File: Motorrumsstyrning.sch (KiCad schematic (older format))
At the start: 60 parts, among them J1 SD_Card_Connector, J10 Jumper, J11 Jumper, J12 Jumper, J13 Jumper, J14 Jumper, J15 Jumper, J16 Jumper, J17 Jumper, J18 Jumper, J19 Jumper, J2 Jumper, J20 Jumper, J21 Jumper, J22 Jumper, J23 Screw_Terminal_01x10, J24 Screw_Terminal_01x10, J3 Jumper, J4 Jumper, J5 Jumper, J6 Jumper, J7 Jumper, J8 Jumper, J9 Jumper, Q1 BC337, Q2 BC337, U1 NUCLEO-F303K8, U2 LM1084-5.0, U3 MCP2551-I-P

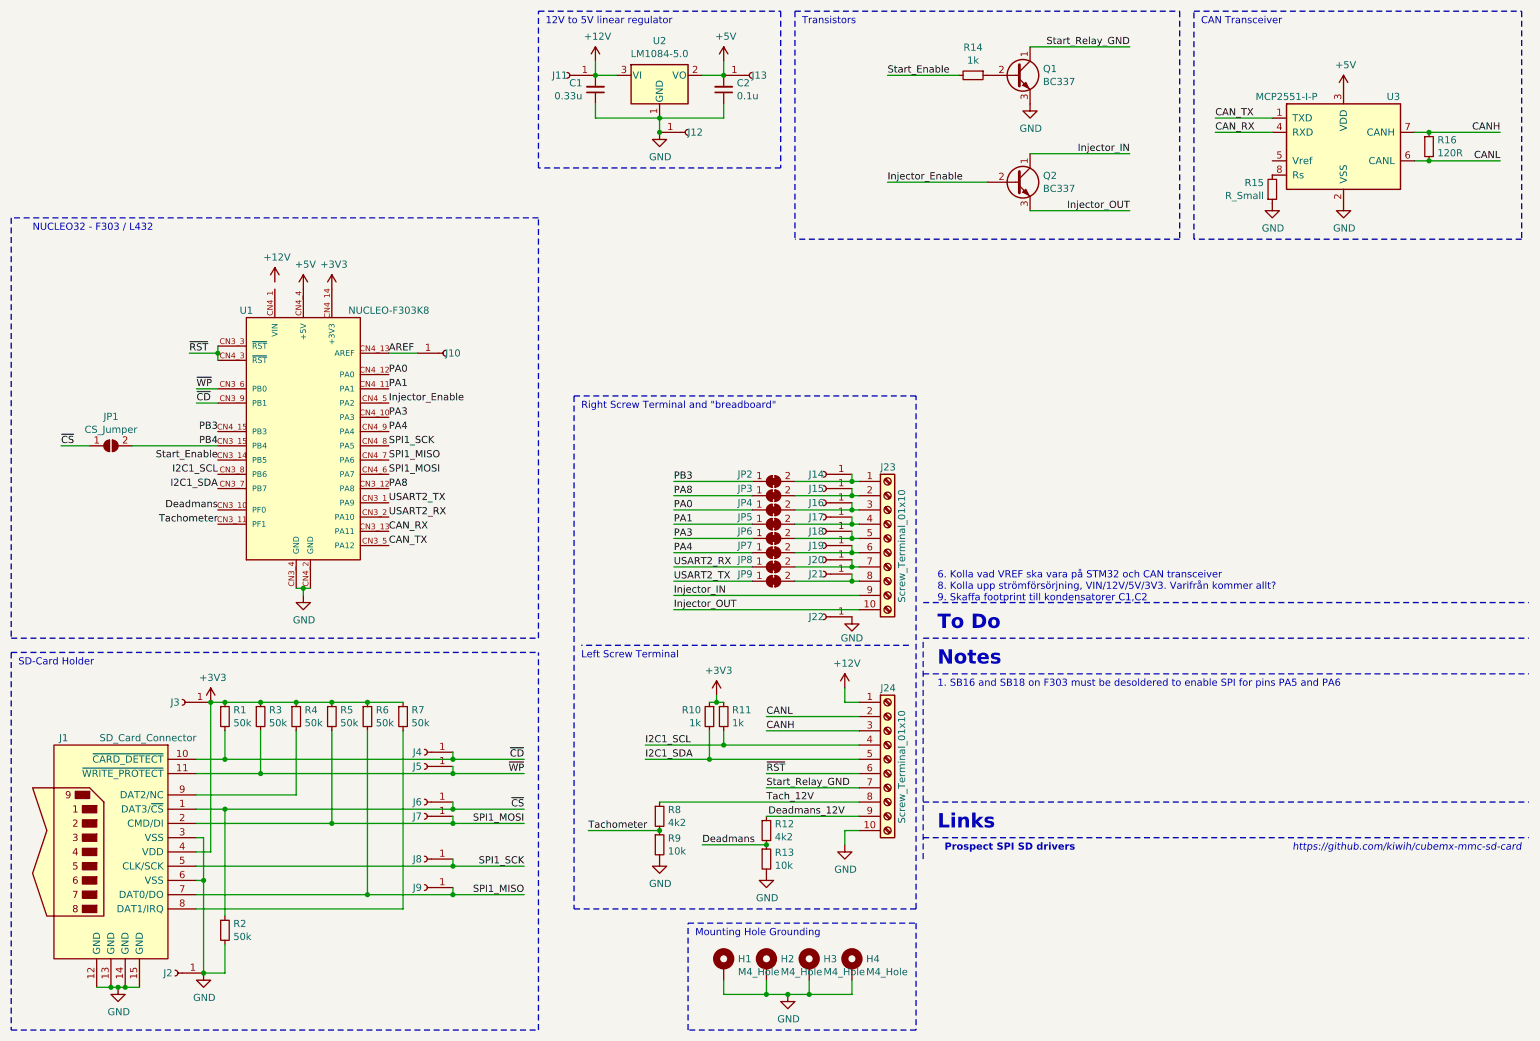
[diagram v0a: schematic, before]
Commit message: Vidareutveckling
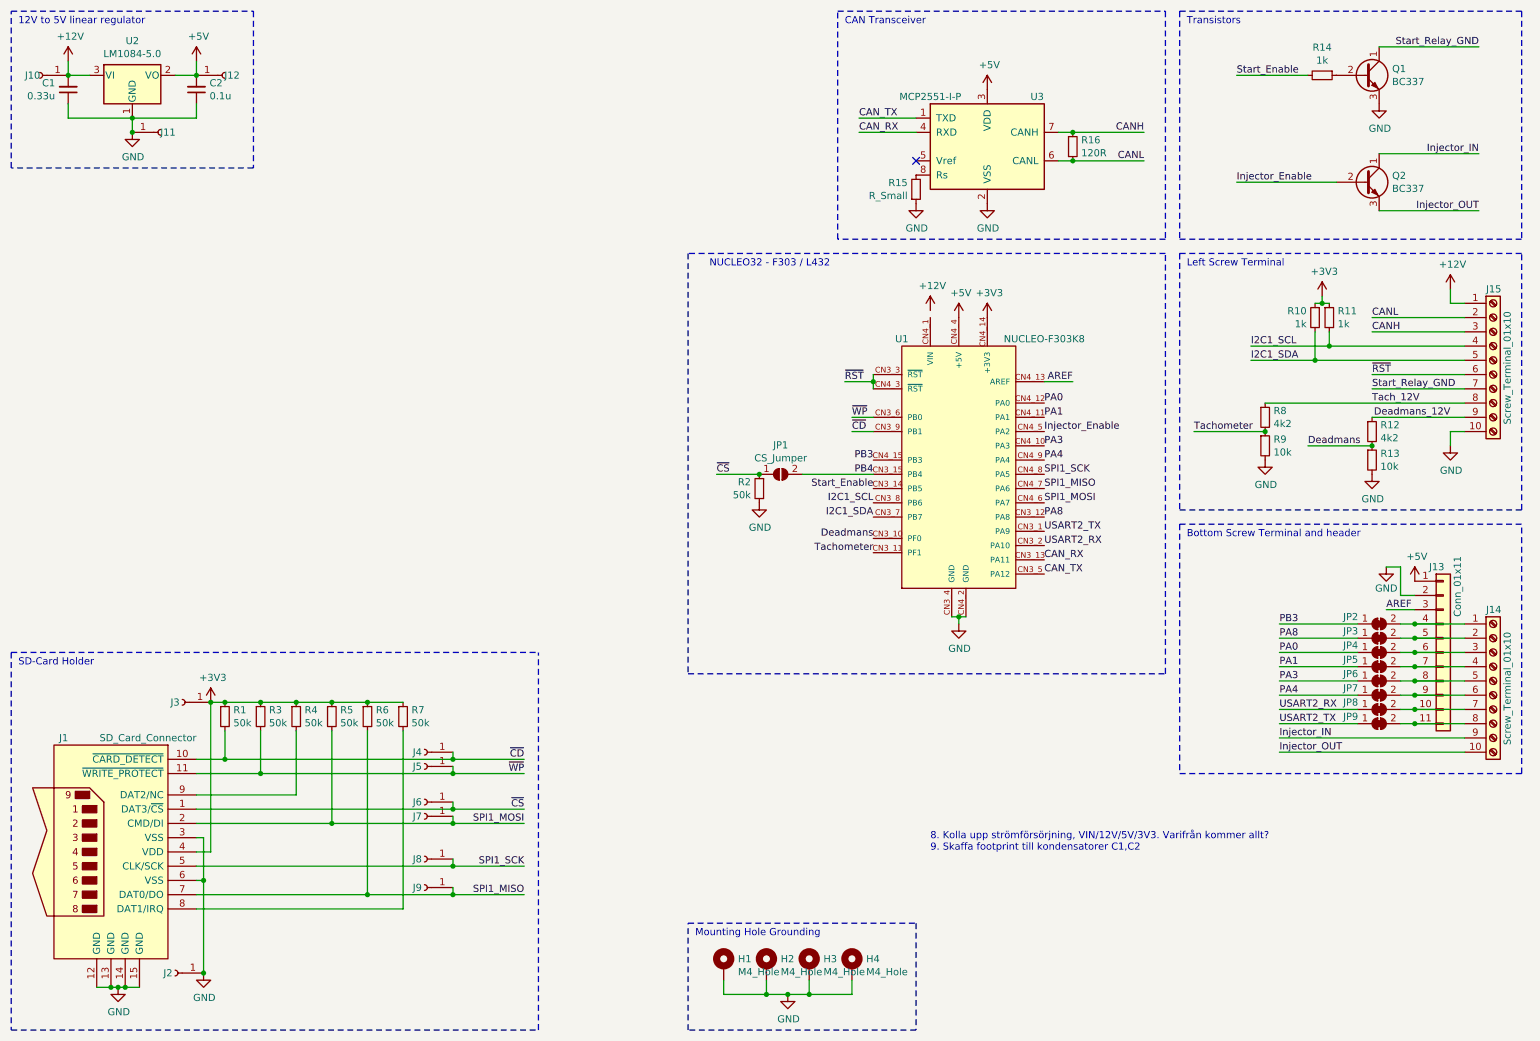
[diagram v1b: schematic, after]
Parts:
- removed J10, J14, J15, J16, J17, J18, J19, J20, J21, J22: Jumper, Vera-MRS-21:THT_Jumper, symbol Connector:Conn_01x01_Female
- added J13: Conn_01x11, Connector_PinHeader_2.54mm:PinHeader_1x11_P2.54mm_Vertical, symbol Connector_Generic:Conn_01x11
- renumbered J11 to J10, J12 to J11, J13 to J12, J23 to J14, J24 to J15
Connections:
- net +5V: now also J13.1 (Pin_1)
- net AREF: now also J13.3 (Pin_3)
- net GND: now also J13.2 (Pin_2)
- net at J14.1 (Pin_1), JP2.2 (B): now also J13.4 (Pin_4)
- net at J14.2 (Pin_2), JP3.2 (B): now also J13.5 (Pin_5)
- net at J14.3 (Pin_3), JP4.2 (B): now also J13.6 (Pin_6)
- net at J14.4 (Pin_4), JP5.2 (B): now also J13.7 (Pin_7)
- net at J14.5 (Pin_5), JP6.2 (B): now also J13.8 (Pin_8)
- net at J14.6 (Pin_6), JP7.2 (B): now also J13.9 (Pin_9)
- net at J14.7 (Pin_7), JP8.2 (B): now also J13.10 (Pin_10)
- net at J14.8 (Pin_8), JP9.2 (B): now also J13.11 (Pin_11)
- no-connect marks 0 -> 1
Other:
- note added: "8. Kolla upp strömförsörjning, VIN/12V/5V/3V3. Varifrån kommer allt? \n9. Skaffa footprint till kondensatorer C1,C2"
- note added: "Bottom Screw Terminal and header"
- note removed: "1. SB16 and SB18 on F303 must be desoldered to enable SPI for pins PA5 and PA6"
- note removed: "6. Kolla vad VREF ska vara på STM32 och CAN transceiver\n8. Kolla upp strömförsörjning, VIN/12V/5V/3V3. Varifrån kommer allt? \n9. Skaffa footprint till kondensatorer C1,C2"
- note removed: "Links"
- note removed: "Notes"
- note removed: "Prospect SPI SD drivers"
- note removed: "Right Screw Terminal and "breadboard""
- note removed: "To Do"
- note removed: "https://github.com/kiwih/cubemx-mmc-sd-card"
- moved on the sheet: C1, C2, J10, J11, J12, J14, J15, JP1, JP2, JP3, JP4, JP5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
